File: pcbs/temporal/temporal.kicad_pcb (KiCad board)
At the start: 2 copper layers, 147.9 x 107.9 mm, 58 parts

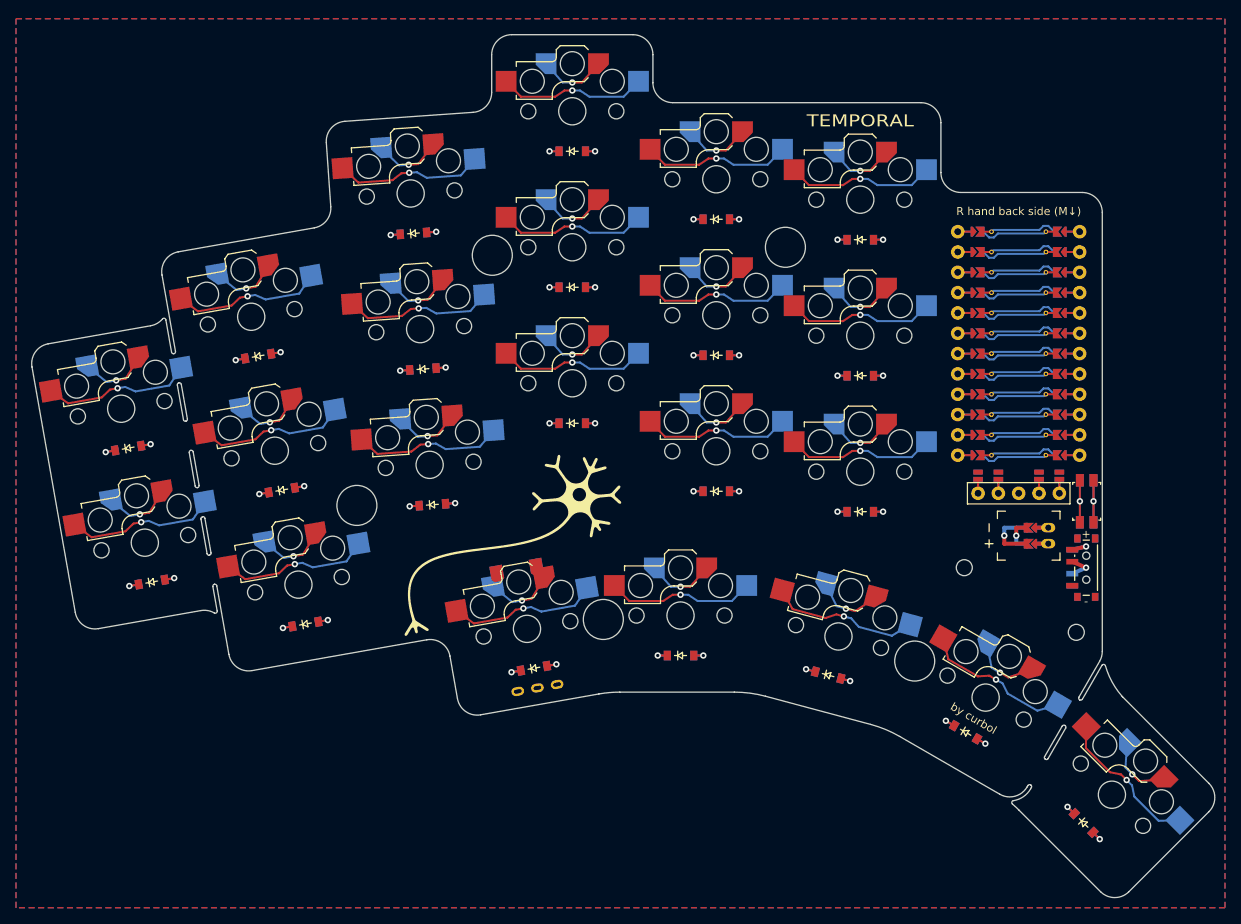
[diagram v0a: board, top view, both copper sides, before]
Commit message: update generated files
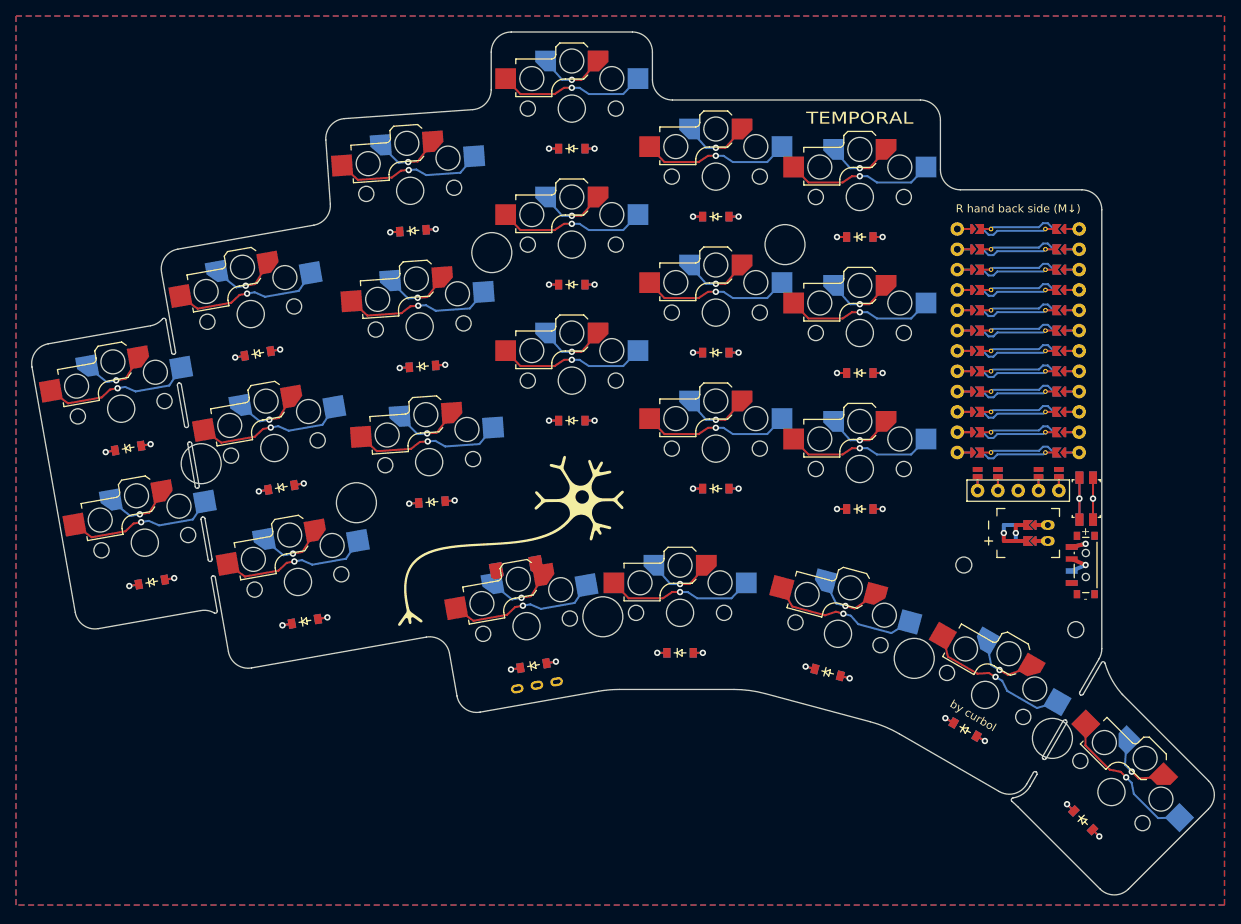
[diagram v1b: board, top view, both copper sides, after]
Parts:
- added MH8: , ceoloide:mounting_hole_npth, F.Cu at (149.4, 86.0)
- added MH9: , ceoloide:mounting_hole_npth, F.Cu at (163.4, 94.1)
- moved MH7 111.4 mm to (54.1, 73.4), turned to 10 degrees
- moved MH6 76.4 mm to (73.5, 78.3), turned to 4 degrees
- moved MH4 58.1 mm to (160.5, 107.7), turned to -30 degrees
- moved MH5 33.7 mm to (104.3, 92.5), turned to 10 degrees
- moved G1 0.34 mm to (92.8, 83.0), turned to 0 degrees
- moved D15 0.34 mm to (136.4, 79.0)
- moved D16 0.34 mm to (136.4, 62.0)
- moved D17 0.34 mm to (136.4, 45.0)
- moved D20 0.34 mm to (132.4, 99.5)
- moved D21 0.34 mm to (149.6, 106.6)
- moved D22 0.34 mm to (164.3, 118.0)
- moved DISP1 0.34 mm to (156.2, 60.0)
- moved JST1 0.34 mm to (159.9, 82.0)
- moved MCU1 0.34 mm to (156.2, 56.7)
- moved MH3 0.34 mm to (143.2, 97.7)
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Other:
- board size 147.9 x 107.9 mm -> 147.8 x 107.9 mm

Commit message: update generated files
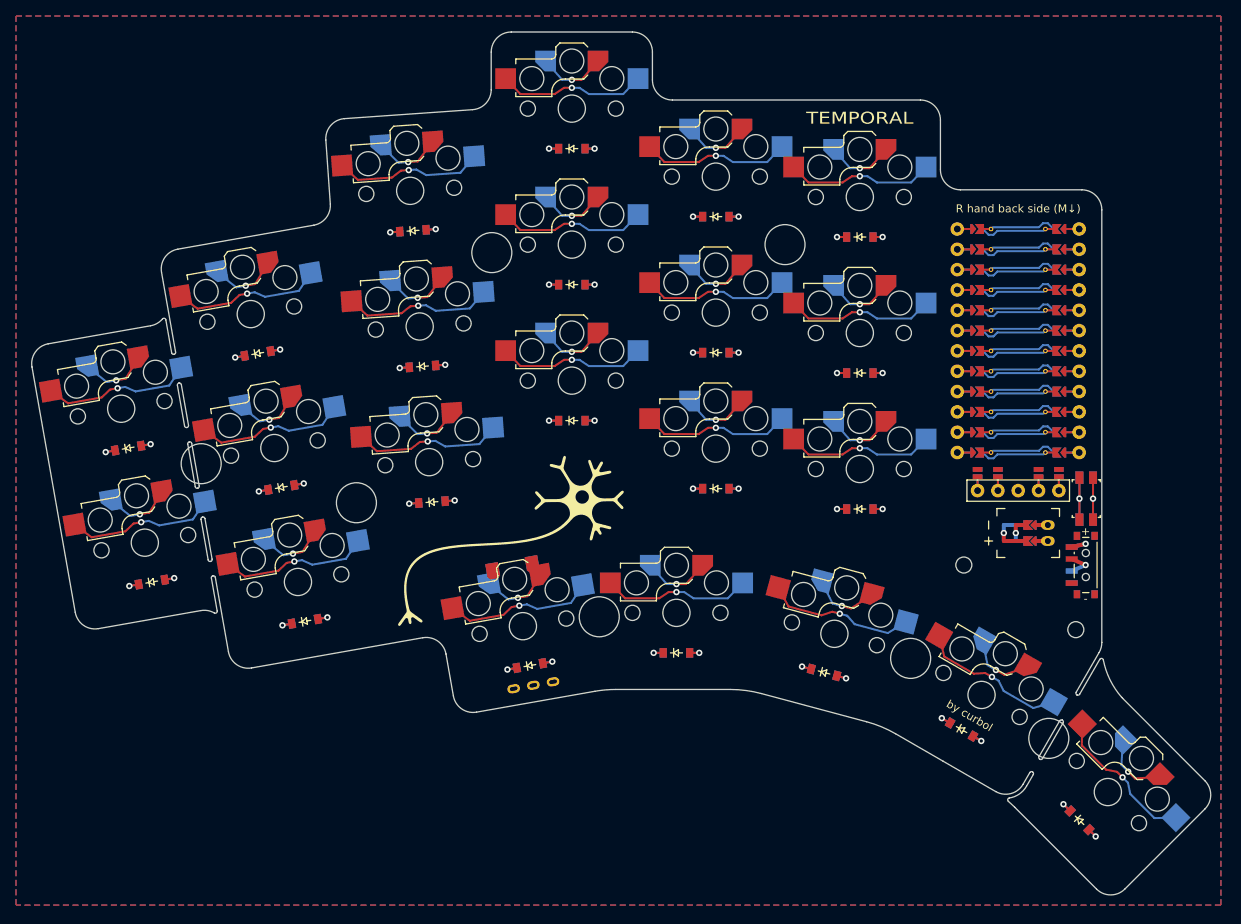
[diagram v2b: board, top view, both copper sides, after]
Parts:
- moved D18 0.45 mm to (95.2, 98.6)
- moved D19 0.45 mm to (113.5, 97.0)
- moved D20 0.45 mm to (132.0, 99.5)
- moved D21 0.45 mm to (149.1, 106.6)
- moved D22 0.45 mm to (163.9, 118.0)
- moved MH3 0.45 mm to (142.8, 97.7)
- moved MH4 0.45 mm to (160.0, 107.7)
- moved MH5 0.45 mm to (103.9, 92.5)
- moved RE1 0.45 mm to (94.3, 93.7)
- moved S18 0.45 mm to (94.3, 93.7)
- moved S19 0.45 mm to (113.5, 92.0)
- moved S20 0.45 mm to (133.2, 94.7)
- moved S21 0.45 mm to (151.6, 102.3)
- moved S22 0.45 mm to (167.4, 114.4)
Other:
- board size 147.8 x 107.9 mm -> 147.4 x 107.9 mm
